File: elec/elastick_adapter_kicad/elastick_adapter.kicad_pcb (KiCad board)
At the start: 2 copper layers, 57.2 x 99.1 mm, 10 parts, among them J1 DE-9JOYSTICK, J2 USB-C Breakout, SW1 POWER, SW2 ROTARY_SWITCH, U1 LOLIN-D32

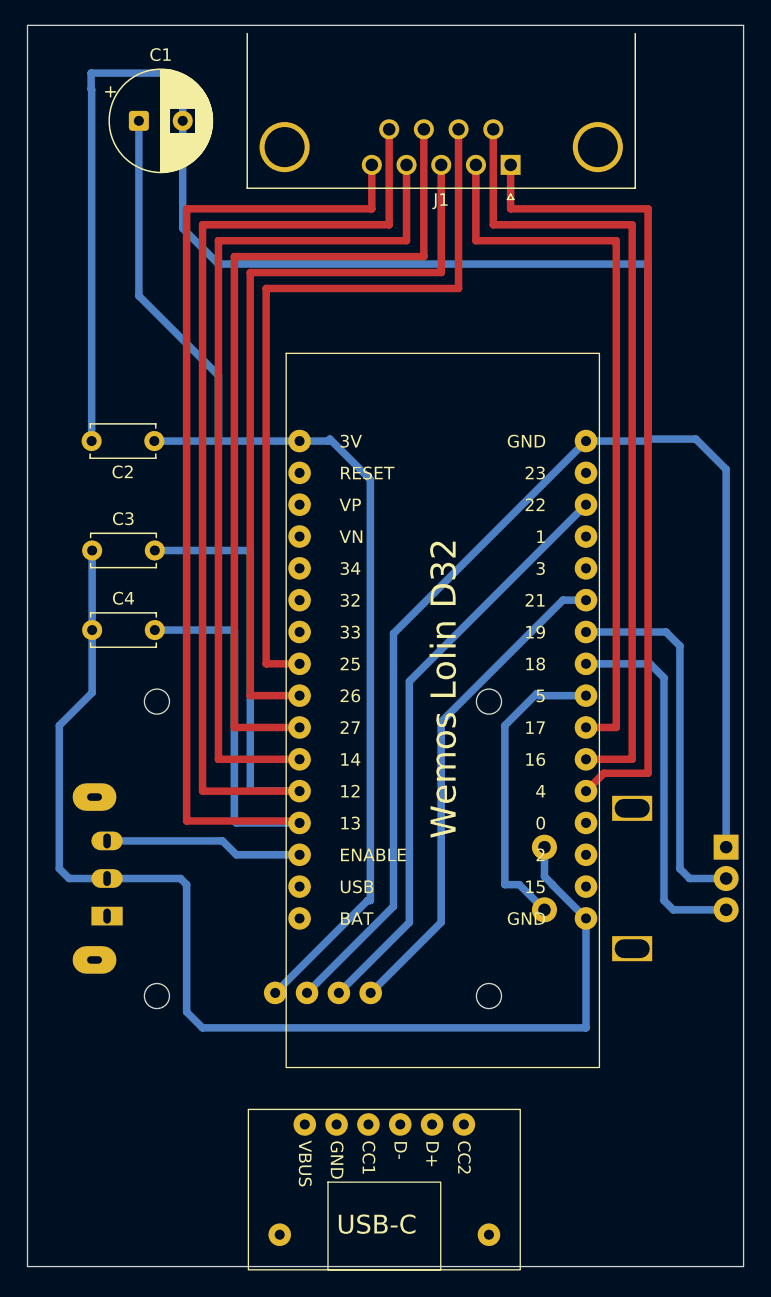
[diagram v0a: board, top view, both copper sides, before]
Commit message: update kicad
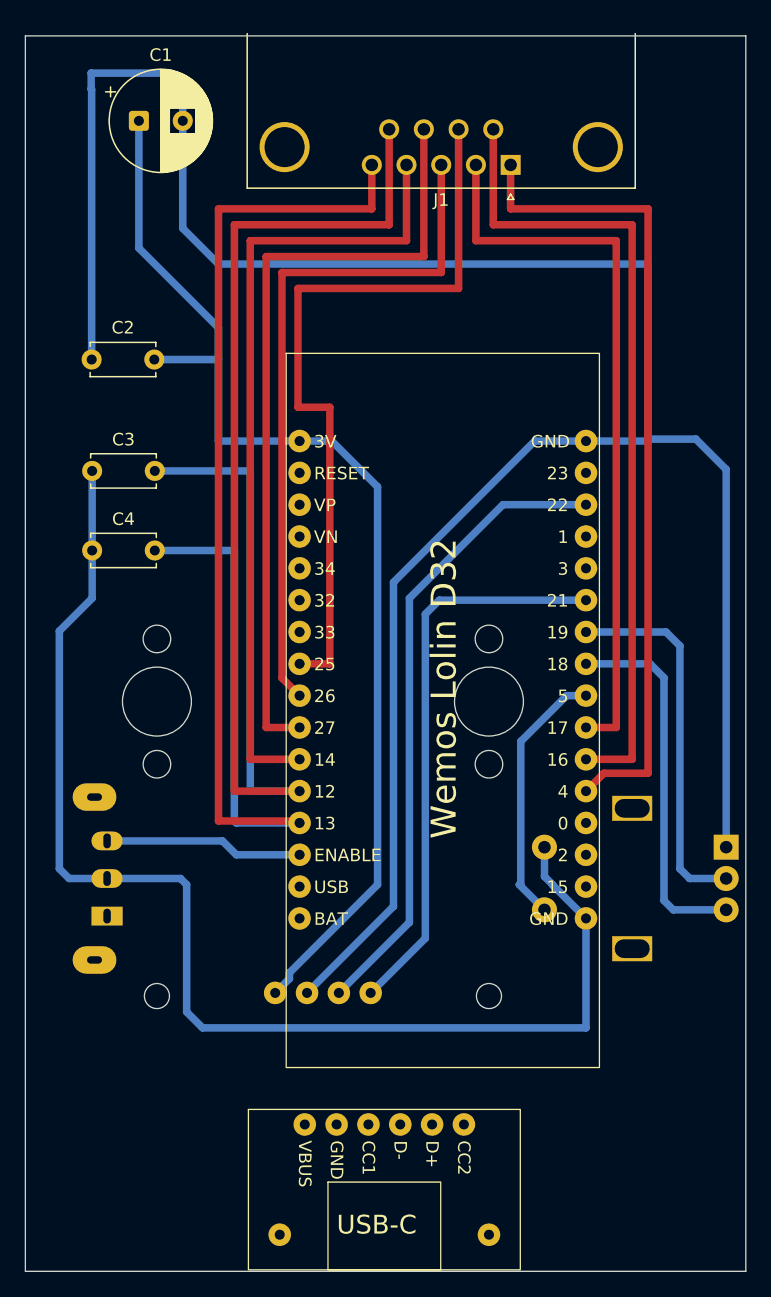
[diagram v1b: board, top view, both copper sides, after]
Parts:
- moved C2 6.51 mm to (115.5, 87.6)
- moved C3 6.35 mm to (110.6, 96.5)
- moved C4 6.35 mm to (110.6, 102.9)
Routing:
- net Net-(U1-26): track 61.5 -> 55.6 mm
- net Net-(DS1-sda): track 39.5 -> 45.3 mm
- net Net-(U1-27): track 68.1 -> 63.0 mm
- net Net-(U1-14): track 68.9 -> 63.8 mm
- net Net-(DS1-scl): track 47.1 -> 51.0 mm
- net Net-(U1-5): track 24.3 -> 21.1 mm
- net Net-(DS1-gnd): track 292.1 -> 294.2 mm
- net Net-(C3-Pad2): track 106.1 -> 107.4 mm
- net Net-(C4-Pad2): track 103.1 -> 104.4 mm
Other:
- board size 57.2 x 99.1 mm -> 57.5 x 98.6 mm
- board text added: "Elastick Adapter 1.0.0"
- board text removed: "Elastick Adapter v1.0.0"
